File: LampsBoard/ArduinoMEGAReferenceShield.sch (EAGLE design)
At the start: 41 parts, among them IC1 LM358N, IC2 LM358N, IC3 5V, Q1 TIP120

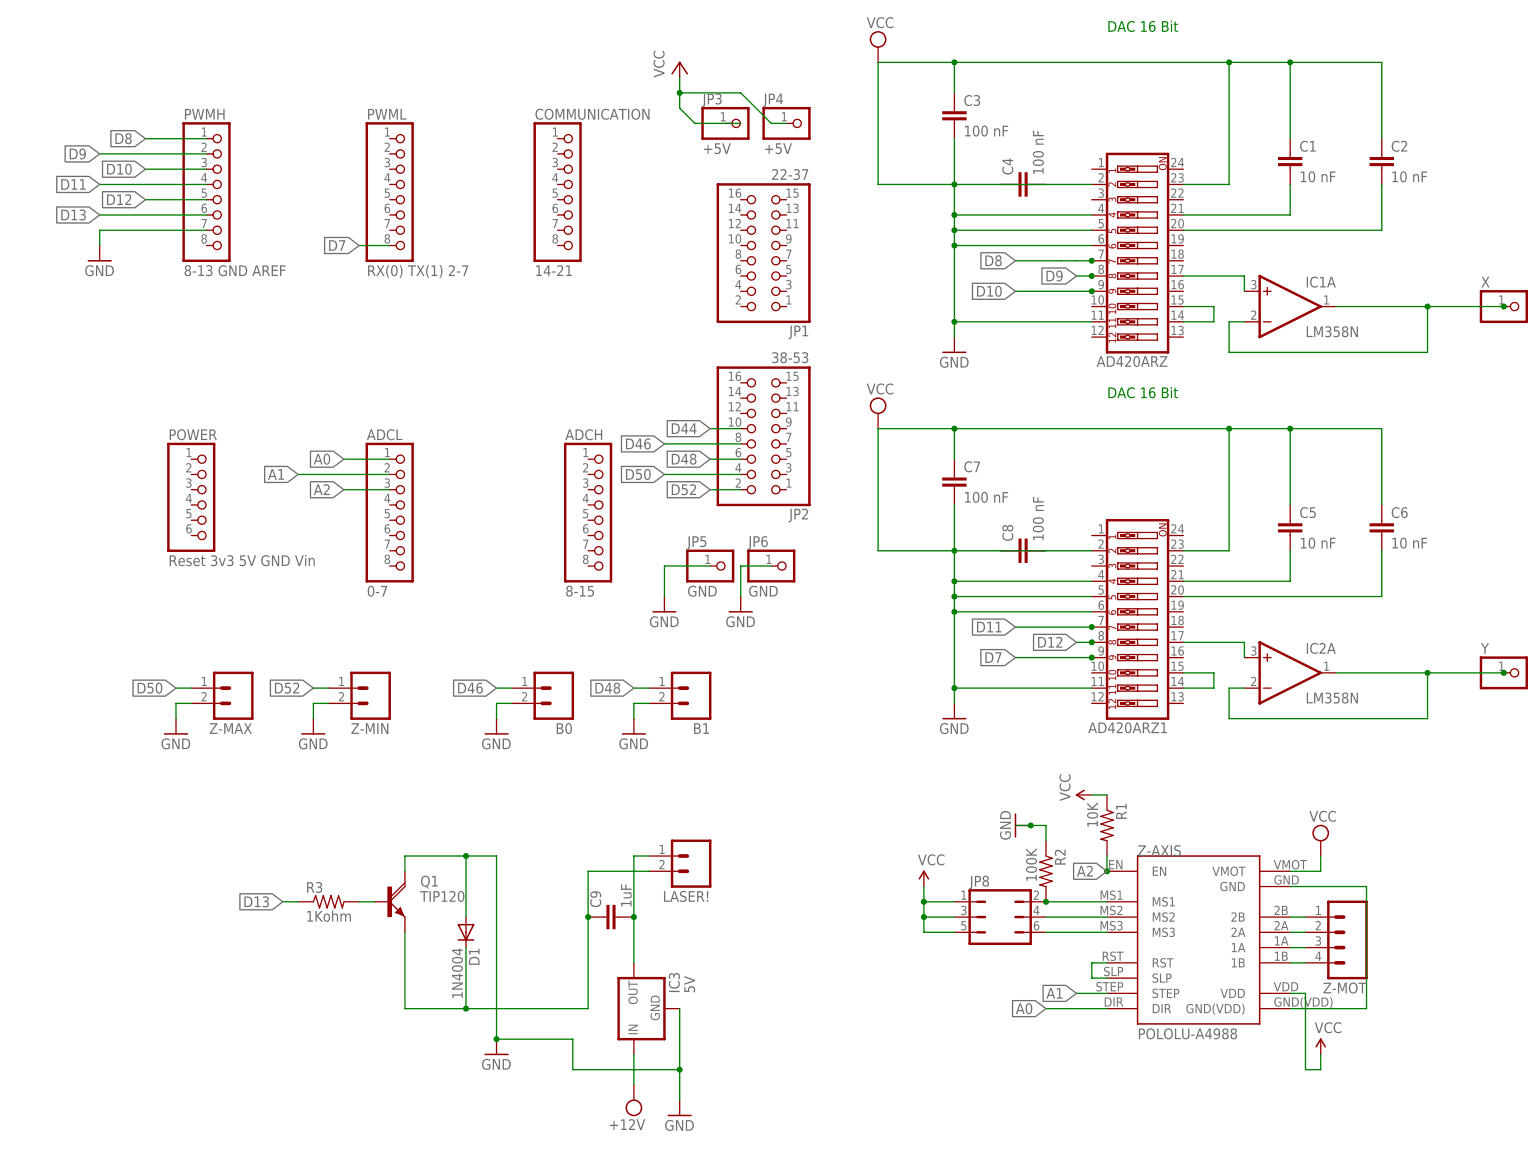
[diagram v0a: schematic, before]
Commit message: Clean up
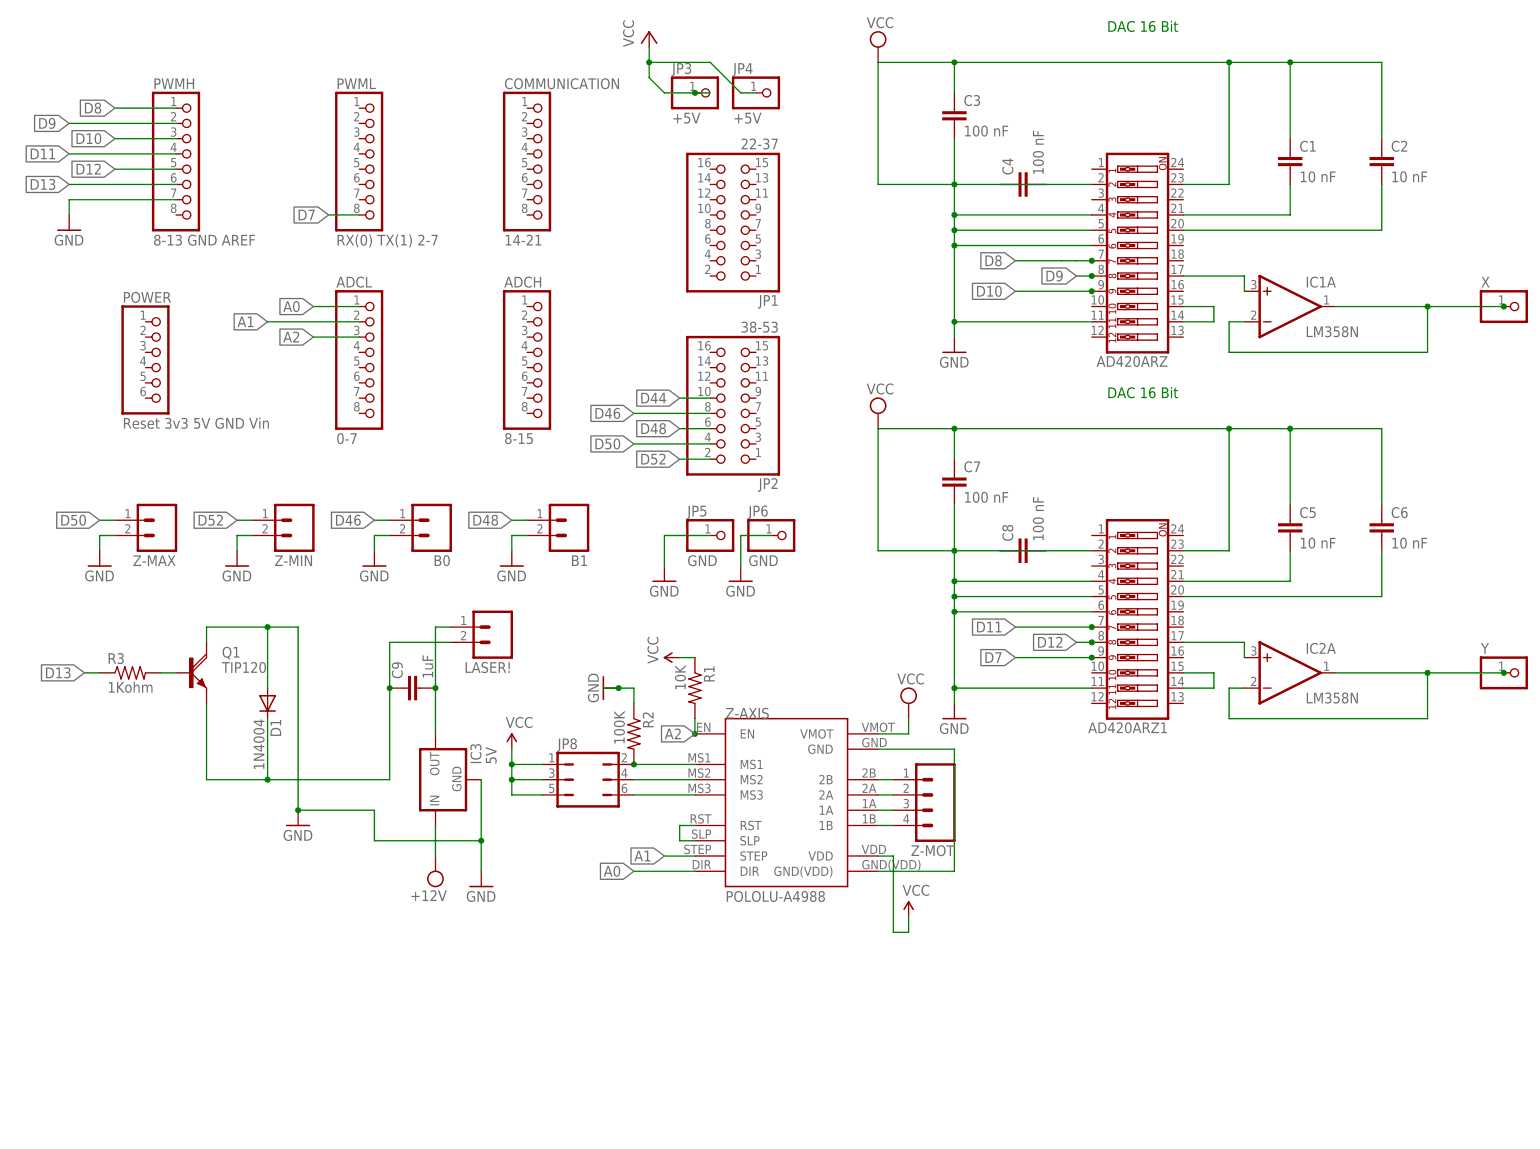
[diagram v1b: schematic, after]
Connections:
- net VCC: now also JP3.1
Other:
- moved on the sheet: ADCH, ADCL, B0, B1, C9, COMMUNICATION, D1, IC3, JP1, JP2, JP3, JP4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
